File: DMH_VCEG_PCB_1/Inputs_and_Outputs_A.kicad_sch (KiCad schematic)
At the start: 13 parts, among them J10 TS_Jack_6.35mm_Sw, J11 TS_Jack_6.35mm_Sw, J12 TS_Jack_6.35mm_Sw, J13 TS_Jack_6.35mm_Sw, J14 TS_Jack_6.35mm_Sw, J201 IDC_02x05, J5 TS_Jack_6.35mm_Sw, J51 Conn_01x06, J6 TS_Jack_6.35mm_Sw, J61 Conn_01x06, J7 TS_Jack_6.35mm_Sw, J8 TS_Jack_6.35mm_Sw, J9 TS_Jack_6.35mm_Sw

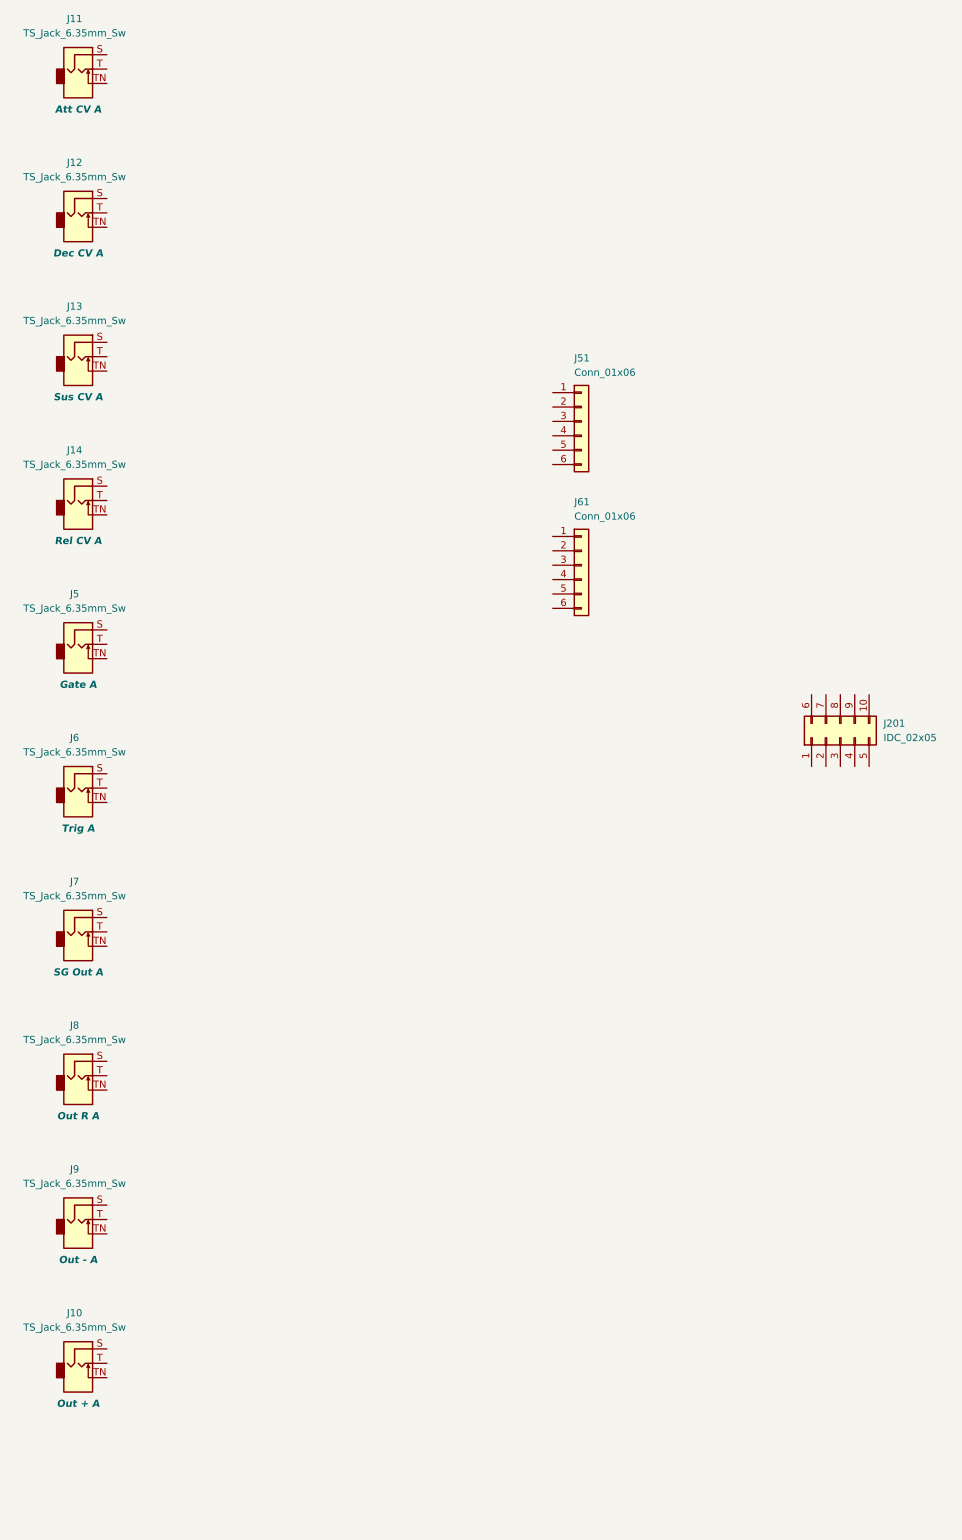
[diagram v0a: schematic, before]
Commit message: IO pages done
Core Circuit A ongoing
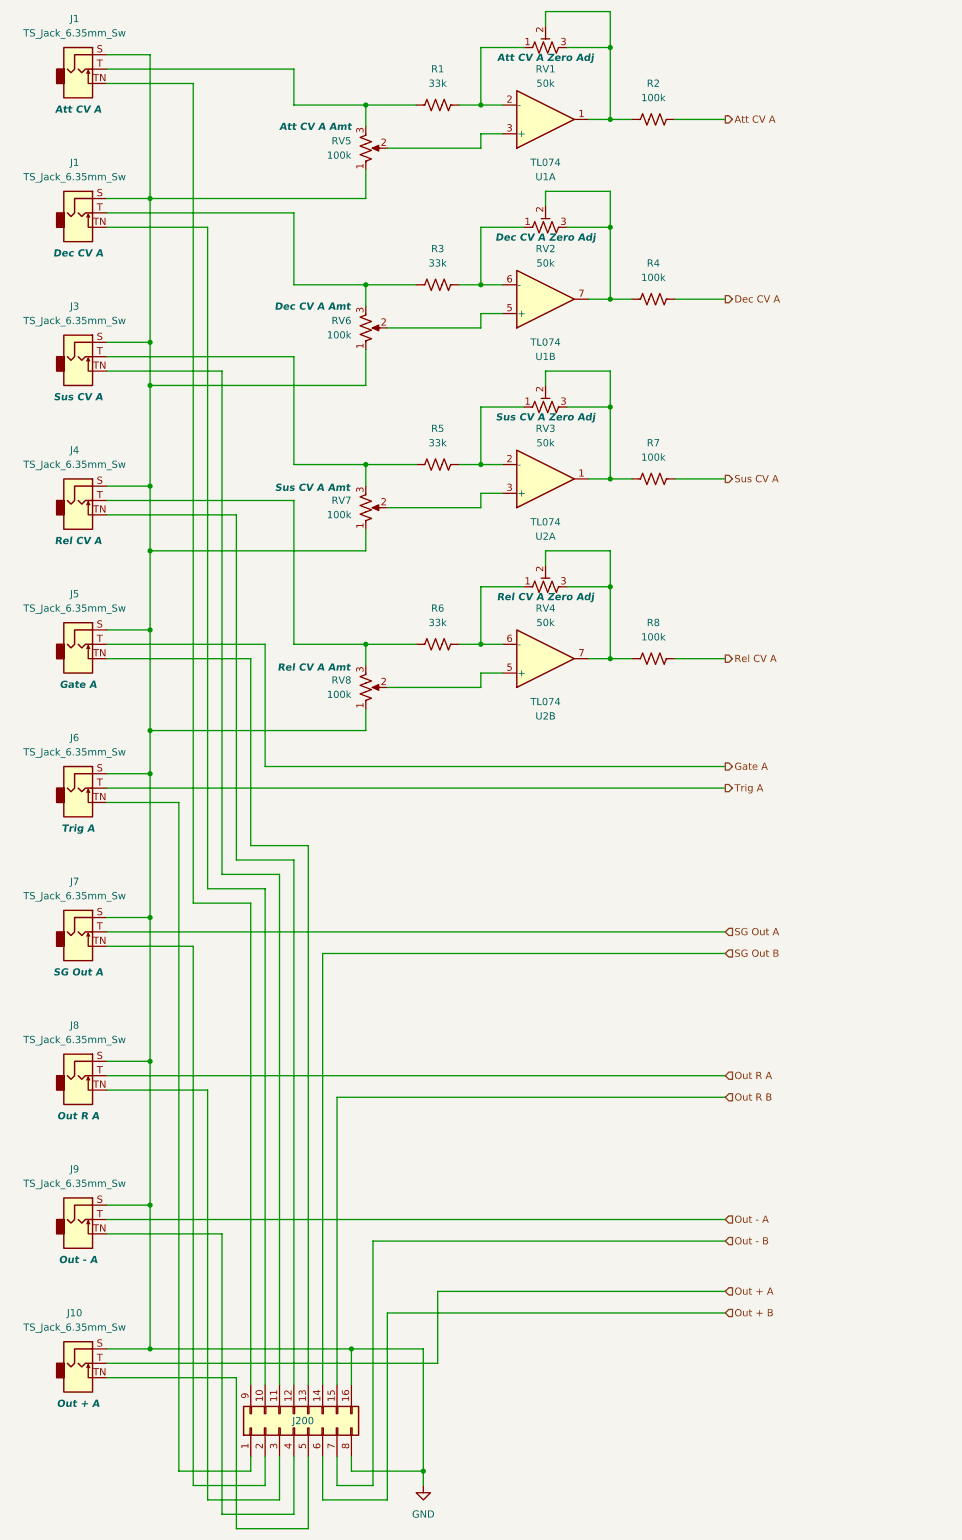
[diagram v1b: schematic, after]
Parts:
- removed J11, J12, J13, J14: TS_Jack_6.35mm_Sw, SynthStuff:CUI_MJ-63052A, symbol SynthStuff:TS_Jack_6.35mm_Sw
- removed J201: IDC_02x05, SynthStuff:IDC-Header_2x05_P2.54mm_Vertical_BackBone, symbol SynthStuff:BackBone_Connector_10Pin
- removed J51, J61: Conn_01x06, Connector_PinSocket_2.54mm:PinSocket_1x06_P2.54mm_Vertical, symbol Connector_Generic:Conn_01x06
- added J1 (x2), J3, J4: TS_Jack_6.35mm_Sw, SynthStuff:CUI_MJ-63052A, symbol SynthStuff:TS_Jack_6.35mm_Sw
- added J200: IDC_02x08, SynthStuff:IDC-Header_2x08_P2.54mm_Vertical_BackBone, symbol SynthStuff:BackBone_Connector_16Pin
- added R1, R3, R5, R6: 33k, Resistor_THT:R_Axial_DIN0207_L6.3mm_D2.5mm_P7.62mm_Horizontal, symbol Device:R_US
- added R2, R4, R7, R8: 100k, Resistor_THT:R_Axial_DIN0207_L6.3mm_D2.5mm_P7.62mm_Horizontal, symbol Device:R_US
- added RV1, RV2, RV3, RV4: 50k, Potentiometer_THT:Potentiometer_Bourns_3296W_Vertical, symbol Device:R_Potentiometer_Trim_US
- added RV5, RV6, RV7, RV8: 100k, SynthStuff:Potentiometer_TT_P110KH1, symbol Device:R_Potentiometer_US
- added U1, U2: TL074, Package_DIP:DIP-14_W7.62mm_Socket, symbol Amplifier_Operational:TL074
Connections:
- net GND: now reaches J8.S
- net GND: now also J10.S, J5.S, J6.S, J7.S, J9.S, J1.S, J1.S, J200.16 (Pin_16), J200.8 (Pin_8), J3.S, J4.S, RV5.1, RV6.1, RV7.1, RV8.1
- net Out R A: now reaches J8.T
- net at J8.TN: now also J200.3 (Pin_3)
- net Gate A: now reaches J5.T
- net at J5.TN: now also J200.13 (Pin_13)
- net Out - A: now reaches J9.T
- net at J9.TN: now also J200.4 (Pin_4)
- net Trig A: now reaches J6.T
- net at J6.TN: now also J200.1 (Pin_1)
- net Out + A: now reaches J10.T
- net at J10.TN: now also J200.5 (Pin_5)
- net SG Out A: now reaches J7.T
- net at J7.TN: now also J200.2 (Pin_2)
- new net: RV8.2, U2.5 (+)
- new net: R6.2, RV4.1, U2.6 (-)
- new net: R8.1, RV4.2, RV4.3, U2.7
- new net: J4.T, R6.1, RV8.3
- new net: J3.T, R5.1, RV7.3
- new net: R5.2, RV3.1, U2.2 (-)
- new net: R7.1, RV3.2, RV3.3, U2.1
- new net: R4.1, RV2.2, RV2.3, U1.7
- new net: R2.1, RV1.2, RV1.3, U1.1
- new net: RV6.2, U1.5 (+)
- new net: J1.T, R3.1, RV6.3
- new net: R3.2, RV2.1, U1.6 (-)
- new net: J1.TN, J200.10 (Pin_10)
- new net: J200.11 (Pin_11), J3.TN
- new net: J200.12 (Pin_12), J4.TN
- new net: J1.TN, J200.9 (Pin_9)
- new net: R1.2, RV1.1, U1.2 (-)
- new net: RV5.2, U1.3 (+)
- new net: J1.T, R1.1, RV5.3
- new net: RV7.2, U2.3 (+)
- new net Att CV A: R2.2
- new net Dec CV A: R4.2
- new net Out + B: J200.6 (Pin_6)
- new net Out - B: J200.7 (Pin_7)
- new net Out R B: J200.15 (Pin_15)
- new net Rel CV A: R8.2
- new net SG Out B: J200.14 (Pin_14)
- new net Sus CV A: R7.2
